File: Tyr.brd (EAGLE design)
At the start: 152.4 x 115.6 mm, 206 parts, among them J1 TYR_TYR_DISPLAY, Q1 DTC123J, SW1 BUTTON, U1 MCP1700T, U2 CONTROLLER_PRTR5V0U2X, U3 STM32F303CC, U4 MB85RC256V, U6 TYR_TPS2552, X1 CONTROLLER_USB-C-12PUSB-C-12P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, Y1 8Mhz

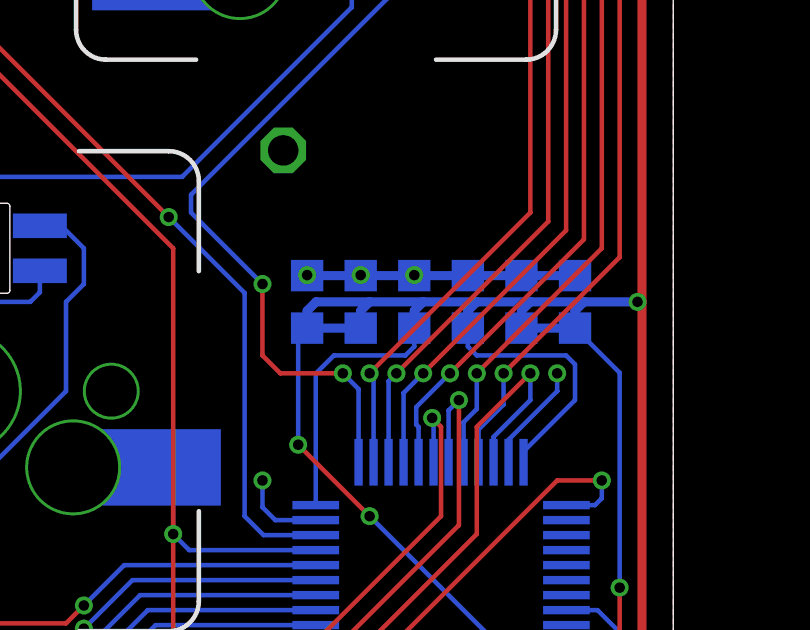
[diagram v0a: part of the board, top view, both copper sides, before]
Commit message: Y branching
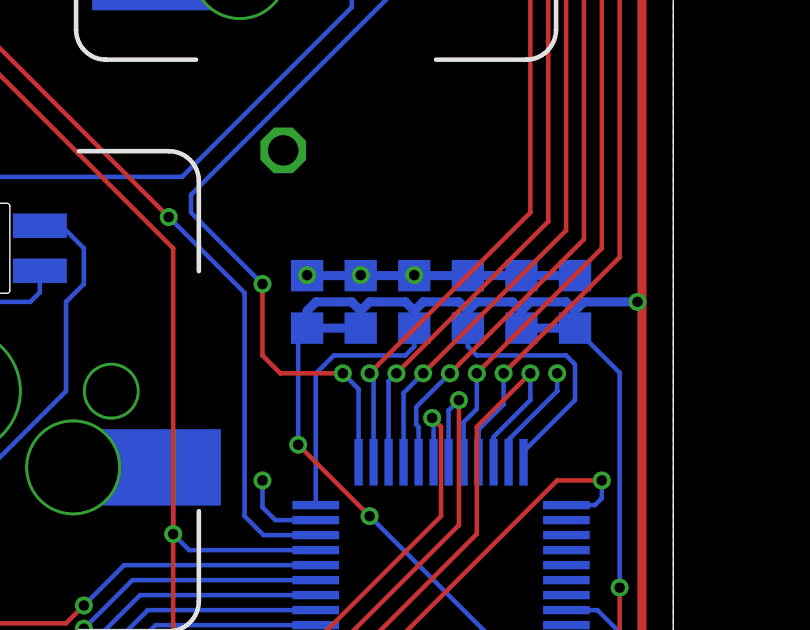
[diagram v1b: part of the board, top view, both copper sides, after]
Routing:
- net 3.3V: track 397.3 -> 396.4 mm
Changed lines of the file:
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@@
 <wire x1="146.0921875" y1="69.74125" x2="145.4071875" y2="69.05625" width="0.3048" layer="16"/>
 <wire x1="151.209375" y1="31.5515625" x2="149.4234375" y2="31.5515625" width="0.3048" layer="16"/>
-<wire x1="149.4234375" y1="31.5515625" x2="147.6375" y2="31.5515625" width="0.3048" layer="16"/>
-<wire x1="147.6375" y1="31.5515625" x2="145.8515625" y2="31.5515625" width="0.3048" layer="16"/>
-<wire x1="145.8515625" y1="31.5515625" x2="144.065625" y2="31.5515625" width="0.3048" layer="16"/>
-<wire x1="144.065625" y1="31.5515625" x2="142.2796875" y2="31.5515625" width="0.3048" layer="16"/>
-<wire x1="142.2796875" y1="31.5515625" x2="140.49375" y2="31.5515625" width="0.3048" layer="16"/>
+<wire x1="148.828125" y1="31.5515625" x2="147.6375" y2="31.5515625" width="0.3048" layer="16"/>
+<wire x1="147.0421875" y1="31.5515625" x2="145.8515625" y2="31.5515625" width="0.3048" layer="16"/>
+<wire x1="145.25625" y1="31.5515625" x2="144.065625" y2="31.5515625" width="0.3048" layer="16"/>
+<wire x1="143.4703125" y1="31.5515625" x2="142.2796875" y2="31.5515625" width="0.3048" layer="16"/>
+<wire x1="141.684375" y1="31.5515625" x2="140.49375" y2="31.5515625" width="0.3048" layer="16"/>
 <wire x1="140.49375" y1="31.5515625" x2="140.19609375" y2="31.25390625" width="0.3048" layer="16"/>
 <wire x1="140.19609375" y1="31.25390625" x2="140.19609375" y2="30.6765625" width="0.3048" layer="16"/>
-<wire x1="141.98203125" y1="30.6765625" x2="141.98203125" y2="31.25390625" width="0.3048" layer="16"/>
 <wire x1="141.98203125" y1="31.25390625" x2="142.2796875" y2="31.5515625" width="0.3048" layer="16"/>
-<wire x1="143.76796875" y1="30.6765625" x2="143.76796875" y2="31.25390625" width="0.3048" layer="16"/>
 <wire x1="143.76796875" y1="31.25390625" x2="144.065625" y2="31.5515625" width="0.3048" layer="16"/>
-<wire x1="145.55390625" y1="30.6765625" x2="145.55390625" y2="31.25390625" width="0.3048" layer="16"/>
 <wire x1="145.55390625" y1="31.25390625" x2="145.8515625" y2="31.5515625" width="0.3048" layer="16"/>
-<wire x1="147.33984375" y1="30.6765625" x2="147.33984375" y2="31.25390625" width="0.3048" layer="16"/>
 <wire x1="147.33984375" y1="31.25390625" x2="147.6375" y2="31.5515625" width="0.3048" layer="16"/>
-<wire x1="149.12578125" y1="30.6765625" x2="149.12578125" y2="31.25390625" width="0.3048" layer="16"/>
 <wire x1="149.12578125" y1="31.25390625" x2="149.4234375" y2="31.5515625" width="0.3048" layer="16"/>
 <wire x1="147.33984375" y1="30.6765625" x2="149.12578125" y2="30.6765625" width="0.3048" layer="16"/>
@@
 <wire x1="118.4671875" y1="7.7390625" x2="115.8875" y2="10.31875" width="0.1524" layer="1"/>
 <wire x1="115.8875" y1="10.31875" x2="115.8875" y2="10.4775" width="0.1524" layer="1"/>
+<wire x1="148.828125" y1="31.5515625" x2="149.12578125" y2="31.25390625" width="0.3048" layer="16"/>
+<wire x1="149.12578125" y1="31.25390625" x2="149.12578125" y2="30.6765625" width="0.3048" layer="16"/>
+<wire x1="147.0421875" y1="31.5515625" x2="147.33984375" y2="31.25390625" width="0.3048" layer="16"/>
+<wire x1="147.33984375" y1="31.25390625" x2="147.33984375" y2="30.6765625" width="0.3048" layer="16"/>
+<wire x1="145.25625" y1="31.5515625" x2="145.55390625" y2="31.25390625" width="0.3048" layer="16"/>
+<wire x1="145.55390625" y1="31.25390625" x2="145.55390625" y2="30.6765625" width="0.3048" layer="16"/>
+<wire x1="143.4703125" y1="31.5515625" x2="143.76796875" y2="31.25390625" width="0.3048" layer="16"/>
+<wire x1="143.76796875" y1="31.25390625" x2="143.76796875" y2="30.6765625" width="0.3048" layer="16"/>
+<wire x1="141.684375" y1="31.5515625" x2="141.98203125" y2="31.25390625" width="0.3048" layer="16"/>
+<wire x1="141.98203125" y1="31.25390625" x2="141.98203125" y2="30.6765625" width="0.3048" layer="16"/>
 </signal>
 <signal name="NRST">
